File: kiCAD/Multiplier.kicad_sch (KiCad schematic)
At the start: 58 parts, among them IC2 ADG1221BRMZ, J1 Conn_01x02_Pin, J2 Conn_01x02_Pin, J3 Conn_01x02_Pin, Q7 Q_Dual_PNP_PNP_C1B1B2C2E2E1, Q8 Q_Dual_PNP_PNP_C1B1B2C2E2E1, U1 TS912, U10 TPS63060, U2 TLV340, U4 TS912, U5 TS912, U6 TS912, U7 TLV340

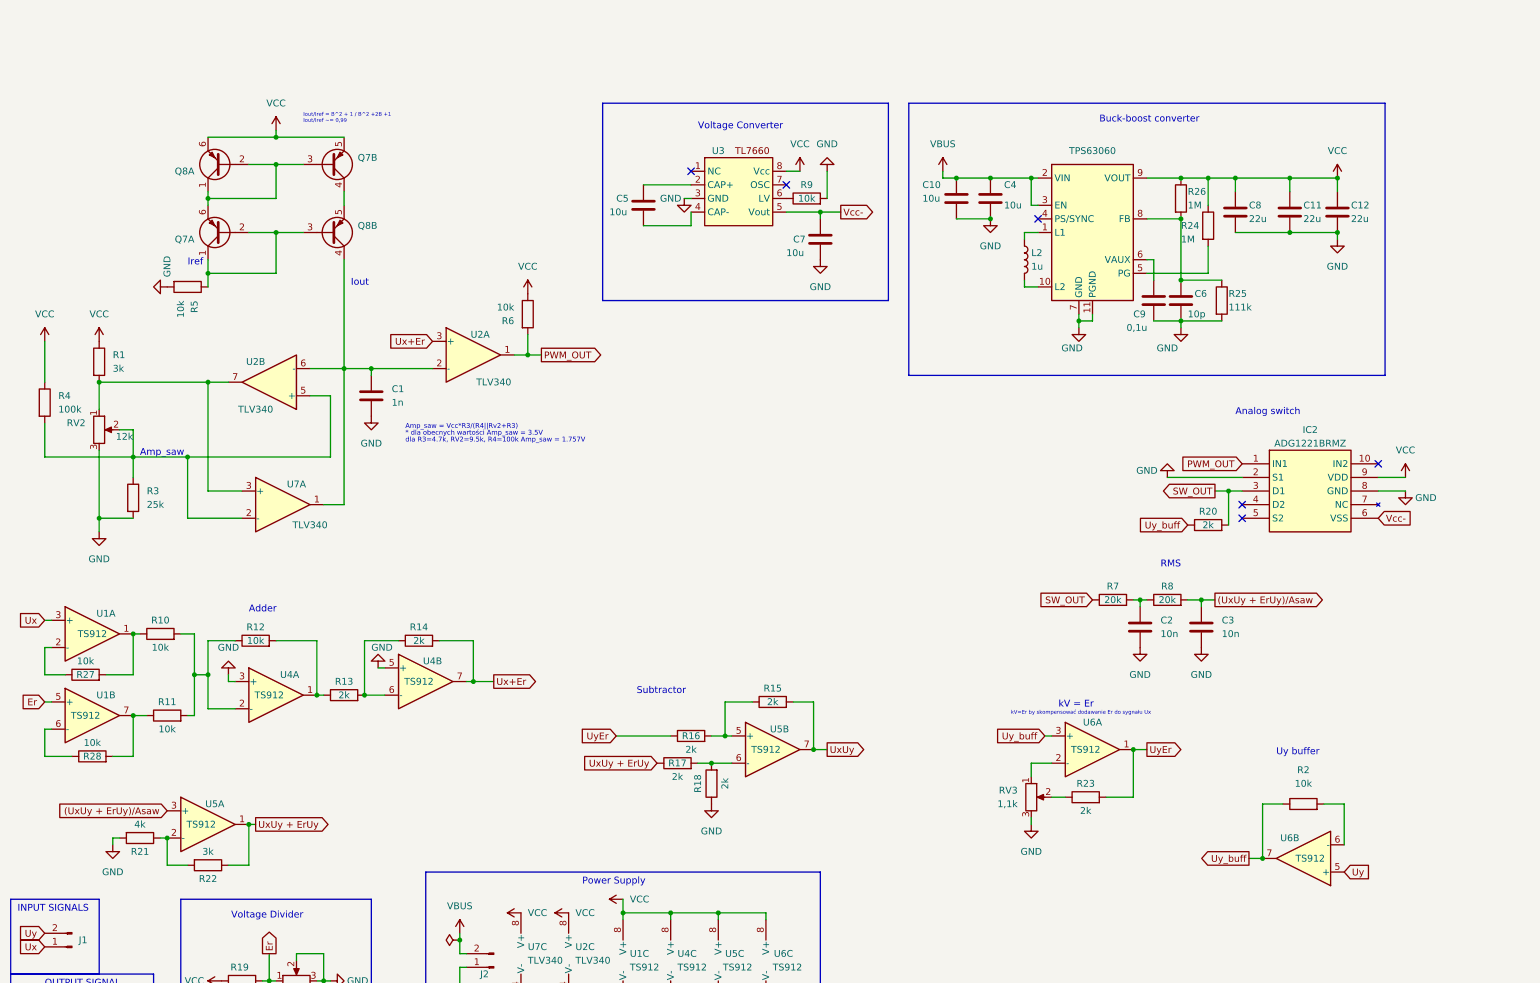
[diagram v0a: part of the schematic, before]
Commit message: adding potentiometer
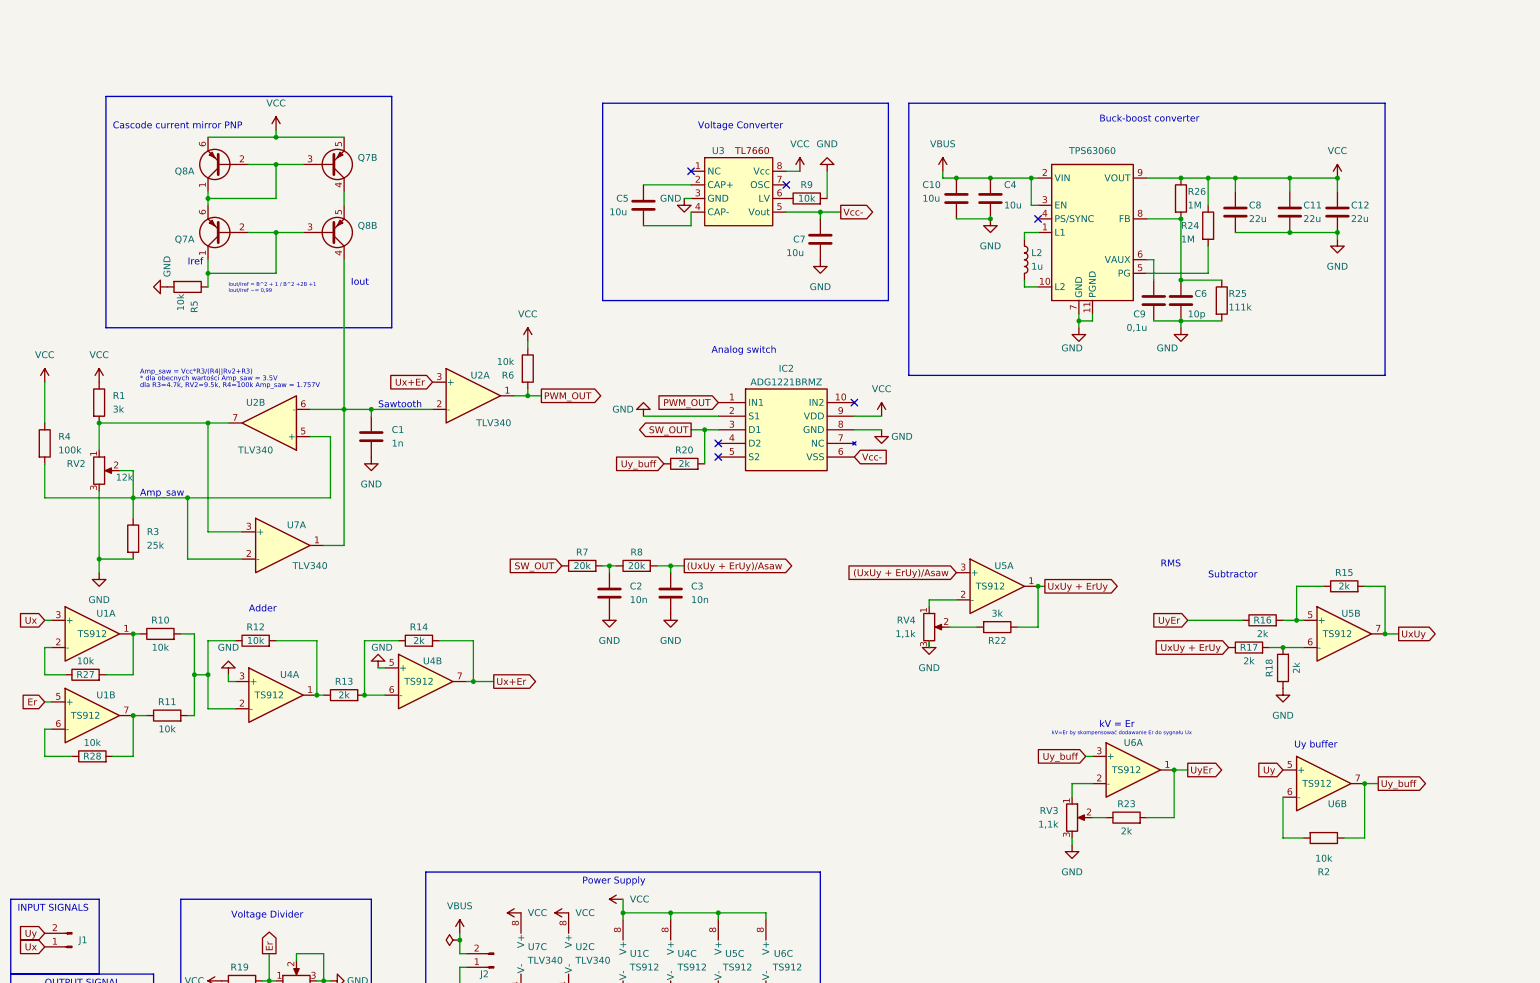
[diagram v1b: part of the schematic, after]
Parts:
- removed R21: 4k, Resistor_SMD:R_0805_2012Metric_Pad1.20x1.40mm_HandSolder, symbol Device:R
- added RV4: 1,1k, Potentiometer_SMD:Potentiometer_Bourns_3314G_Vertical, symbol Device:R_Potentiometer
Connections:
- net GND: now also RV4.3
- net at U5.2 (-): now also RV4.1; no longer R22.2
- new net: R22.2, RV4.2
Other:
- note added: "Cascode current mirror PNP"
- note added: "Sawtooth"
- moved on the sheet: C1, C2, C3, IC2, R1, R15, R16, R17, R18, R2, R20, R22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
